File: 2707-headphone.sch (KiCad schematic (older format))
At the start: 24 parts, among them SW1 SPST, SW2 SPST, SW3 SPST, SW4 SPST, SW5 SPST, SW6 SPST, SW7 SPST, U1 PCM2707, X1 CRYSTAL, X2 USB-B-H

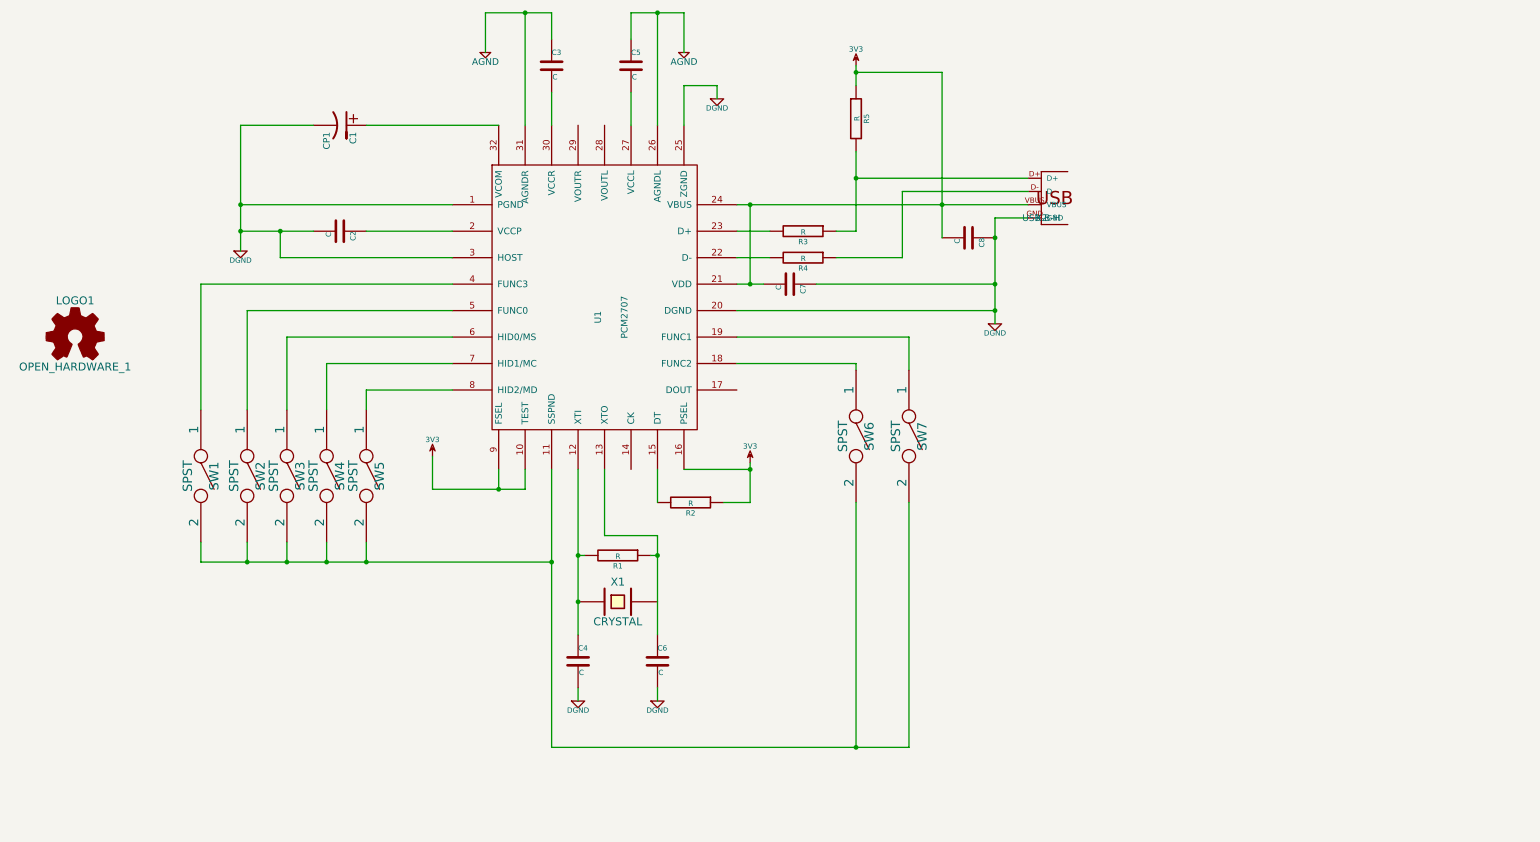
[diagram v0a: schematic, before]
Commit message: made hierarchy
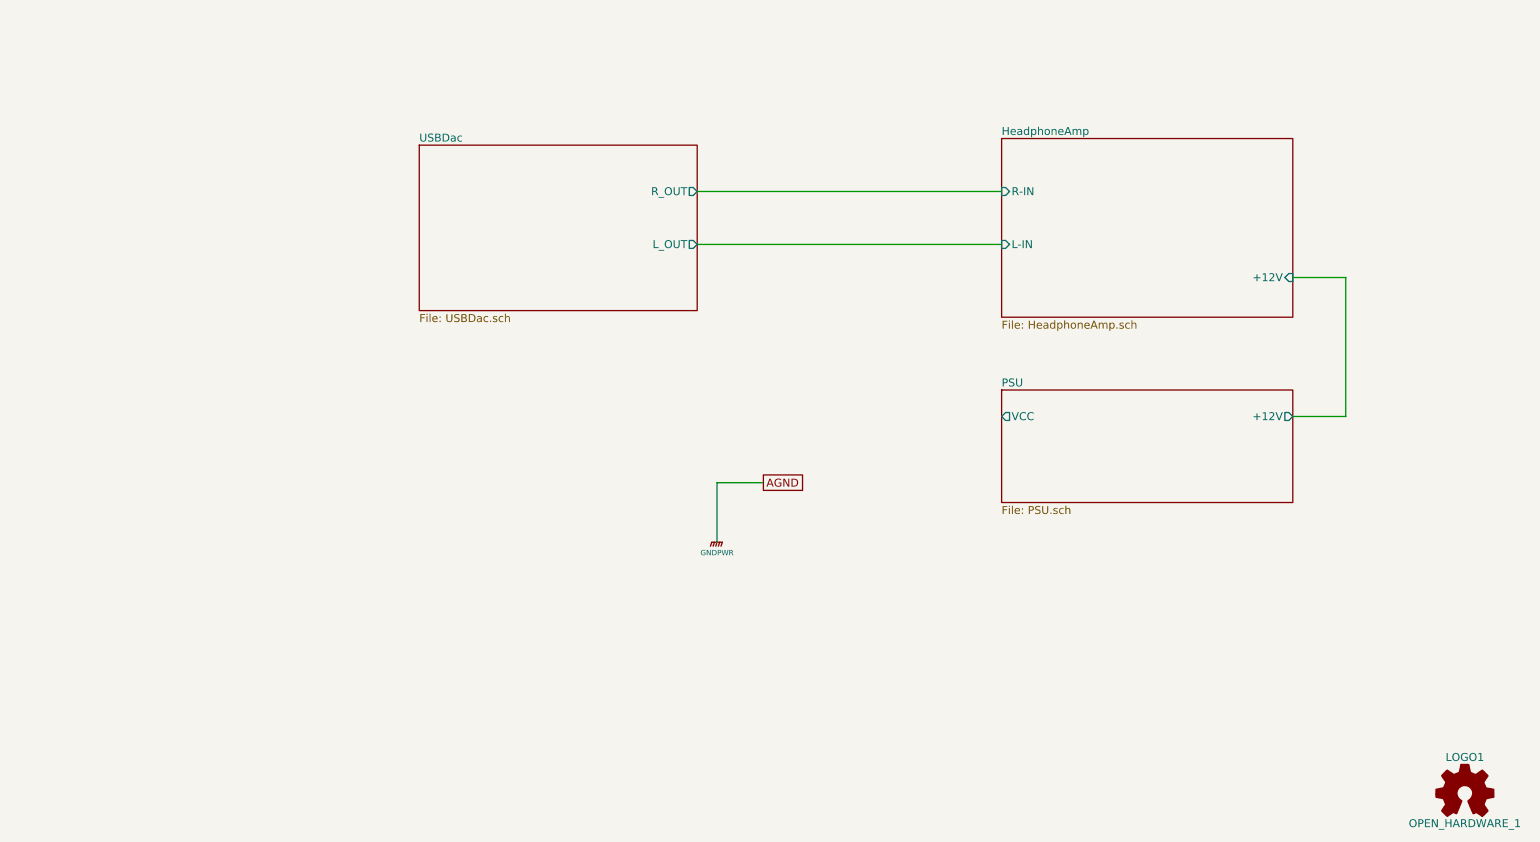
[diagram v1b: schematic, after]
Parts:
- removed C1: CP1, symbol CP1
- removed C2, C3, C4, C5, C6, C7, C8: C, symbol C
- removed R1, R2, R3, R4, R5: R, symbol R
- removed SW1, SW2, SW3, SW4, SW5, SW6, SW7: SPST, symbol SPST
- removed U1: PCM2707, SMD_Packages:TQFP32, symbol PCM2707
- removed X1: CRYSTAL, symbol CRYSTAL
- removed X2: USB-B-H, con-usb-USB-B-H, symbol USB-B-H
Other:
- moved on the sheet: LOGO1
